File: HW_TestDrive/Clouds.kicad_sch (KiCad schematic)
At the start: 11 parts, among them J1 Conn_01x10, J2 Conn_01x04, U1 AS5600L-ASOM, U2 DRV8313PWPR

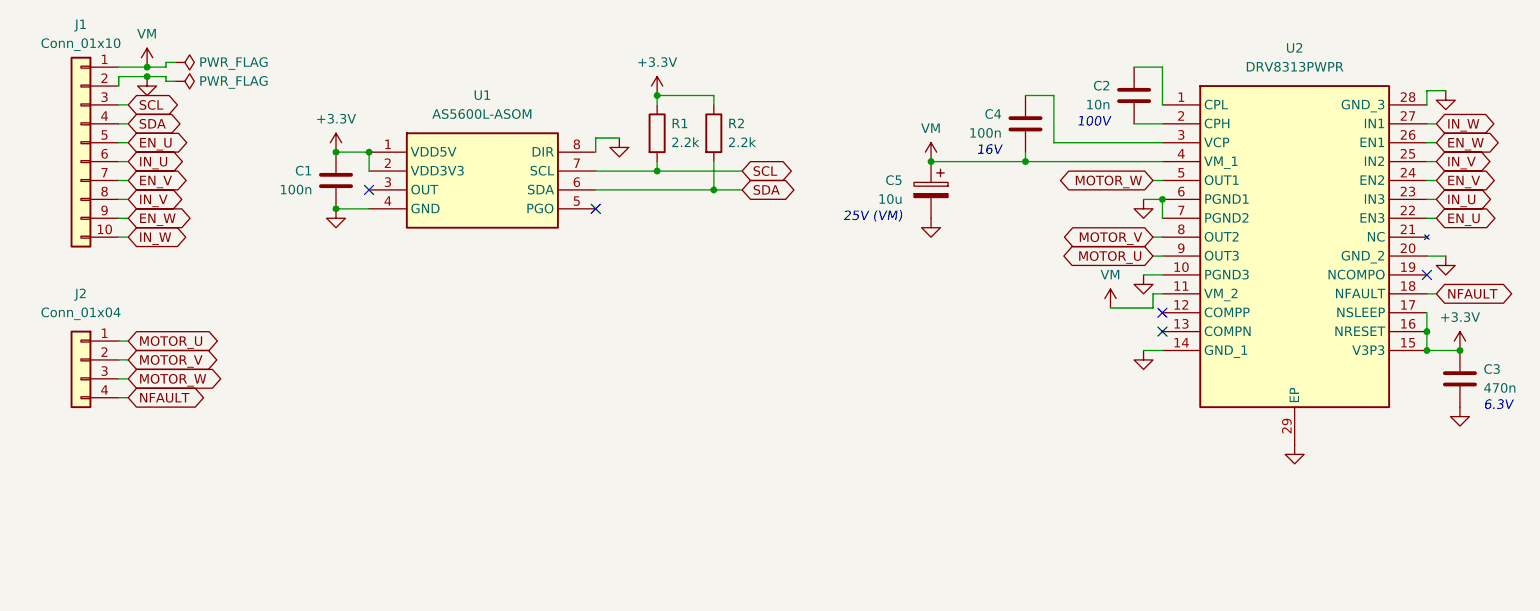
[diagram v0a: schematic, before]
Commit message: Revise schematic
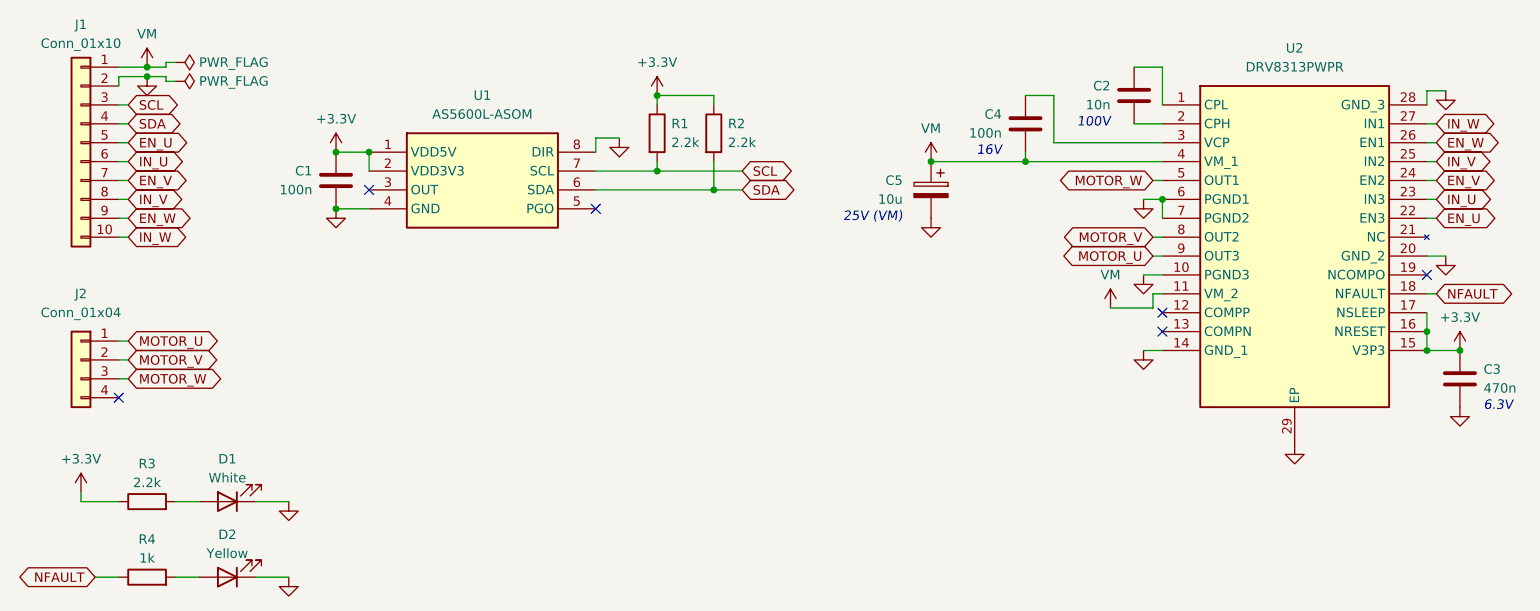
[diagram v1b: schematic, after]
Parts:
- added D1: White, LED_SMD:LED_0805_2012Metric, symbol Device:LED
- added D2: Yellow, LED_SMD:LED_0805_2012Metric, symbol Device:LED
- added R3: 2.2k, Resistor_SMD:R_0603_1608Metric, symbol Device:R
- added R4: 1k, Resistor_SMD:R_0603_1608Metric, symbol Device:R
- C1, C2, C3, C4: footprint (none) -> Capacitor_SMD:C_0603_1608Metric
- C5: footprint (none) -> Capacitor_SMD:CP_Elec_5x3.9
- J1: footprint (none) -> Connector_PinHeader_2.54mm:PinHeader_1x10_P2.54mm_Vertical
- J2: footprint (none) -> Connector_PinHeader_2.54mm:PinHeader_1x04_P2.54mm_Vertical
- R1, R2: footprint (none) -> Resistor_SMD:R_0603_1608Metric
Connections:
- net +3.3V: now also R3.1
- net GND: now also D1.1 (K), D2.1 (K)
- net NFAULT: now also R4.1; no longer J2.4 (Pin_4)
- new net: D2.2 (A), R4.2
- new net: D1.2 (A), R3.2
- no-connect marks 5 -> 6
